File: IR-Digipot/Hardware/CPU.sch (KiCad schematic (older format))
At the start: 14 parts, among them J1 Conn_1x06_Generic, J2 Conn_1x03_Generic, U1 PIC18F2550T-I/SO, U2 TCM809, U3 TSOP754, X1 20 MHz

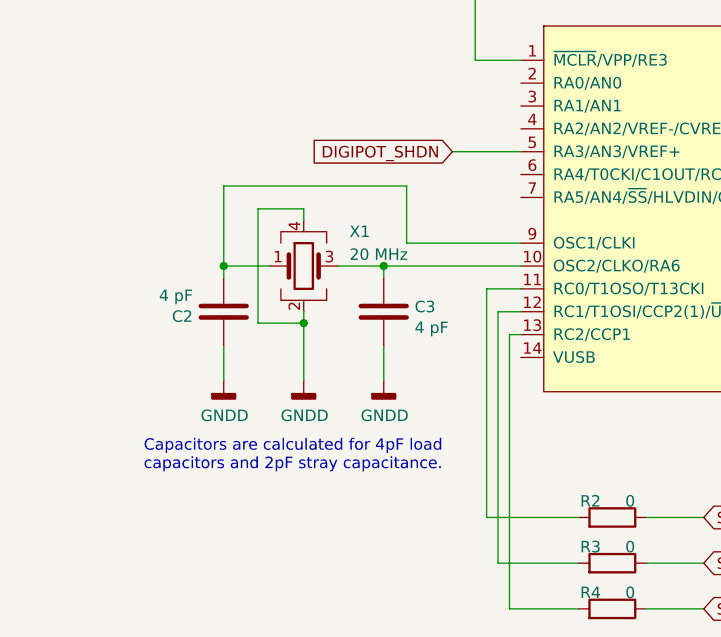
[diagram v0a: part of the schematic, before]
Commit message: Wire high-side switch FET for +5VA
The PIC port should be able to draw enough current to
properly control the switch.
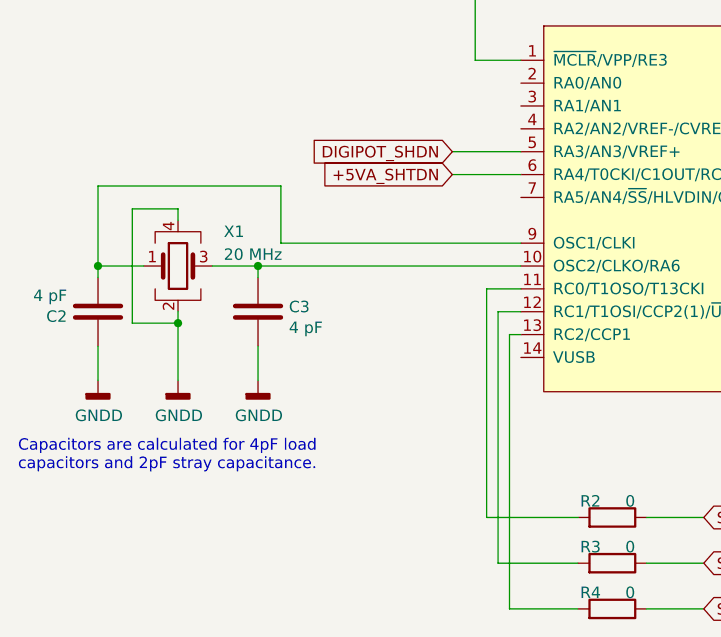
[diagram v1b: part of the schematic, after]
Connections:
- net +5VA_SHTDN: now reaches U1.6 (RA4/T0CKI/C1OUT/RCV)
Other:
- moved on the sheet: C2, C3, X1
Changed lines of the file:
@@
 L Library:Crystal_GND24 X1
 U 1 1 5FE286DC
-P 2300 3600
-F 0 "X1" H 2500 3750 50  0000 L CNN
-F 1 "20 MHz" H 2500 3650 50  0000 L CNN
-F 2 "Librray:Crystal_SMD_4Pin_3.2x2.5mm" H 2700 3600 50  0001 C CNN
-F 3 "${KIPRJMOD}/../../Datasheet/ABM10W SERIES IoT OPTIMIZED LOW PROFILE QUARTZ CRYSTAL.pdf" H 2700 3600 50  0001 C CNN
-F 4 "CRYSTAL 20.0000MHZ 4PF SMD" H 2300 3600 50  0001 C CNN "Description"
-F 5 "Abracon LLC" H 2300 3600 50  0001 C CNN "Manufacturer"
-F 6 "ABM8W-20.0000MHZ-4-K1Z-T3" H 2300 3600 50  0001 C CNN "Manufacturer Part Number"
-F 7 "535-14037-1-ND" H 2300 3600 50  0001 C CNN "Digi-Key Part Number"
-	1    2300 3600
-	1    0    0    -1
-$EndComp
-Wire Wire Line
-	3250 3500 2750 3500
-Wire Wire Line
-	2750 3500 2750 3250
+P 1750 3600
+F 0 "X1" H 1950 3750 50  0000 L CNN
+F 1 "20 MHz" H 1950 3650 50  0000 L CNN
+F 2 "Librray:Crystal_SMD_4Pin_3.2x2.5mm" H 2150 3600 50  0001 C CNN
+F 3 "${KIPRJMOD}/../../Datasheet/ABM10W SERIES IoT OPTIMIZED LOW PROFILE QUARTZ CRYSTAL.pdf" H 2150 3600 50  0001 C CNN
+F 4 "CRYSTAL 20.0000MHZ 4PF SMD" H 1750 3600 50  0001 C CNN "Description"
+F 5 "Abracon LLC" H 1750 3600 50  0001 C CNN "Manufacturer"
+F 6 "ABM8W-20.0000MHZ-4-K1Z-T3" H 1750 3600 50  0001 C CNN "Manufacturer Part Number"
+F 7 "535-14037-1-ND" H 1750 3600 50  0001 C CNN "Digi-Key Part Number"
+	1    1750 3600
+	1    0    0    -1
+$EndComp
+Wire Wire Line
+	2200 3500 2200 3250
 $Comp
 L Library:C C3
 U 1 1 5FE2C5B6
-P 2650 3800
-F 0 "C3" V 2671 3665 50  0000 R CNN
-F 1 "4 pF" V 2580 3665 50  0000 R CNN
-F 2 "Librray:C_0402_1005Metric" H 2500 4000 50  0001 C CNN
-F 3 "" H 2500 4000 50  0001 C CNN
-F 4 "CAP CER 4PF 50V C0G/NP0 0402" V 2650 3800 50  0001 C CNN "Description"
-F 5 "KEMET" V 2650 3800 50  0001 C CNN "Manufacturer"
-F 6 "CBR04C409B5GAC" V 2650 3800 50  0001 C CNN "Manufacturer Part Number"
-F 7 "399-13246-1-ND" V 2650 3800 50  0001 C CNN "Digi-Key Part Number"
-	1    2650 3800
+P 2100 3800
+F 0 "C3" V 2121 3665 50  0000 R CNN
+F 1 "4 pF" V 2030 3665 50  0000 R CNN
+F 2 "Librray:C_0402_1005Metric" H 1950 4000 50  0001 C CNN
+F 3 "" H 1950 4000 50  0001 C CNN
+F 4 "CAP CER 4PF 50V C0G/NP0 0402" V 2100 3800 50  0001 C CNN "Description"
+F 5 "KEMET" V 2100 3800 50  0001 C CNN "Manufacturer"
+F 6 "CBR04C409B5GAC" V 2100 3800 50  0001 C CNN "Manufacturer Part Number"
+F 7 "399-13246-1-ND" V 2100 3800 50  0001 C CNN "Digi-Key Part Number"
+	1    2100 3800
 	0    -1   -1   0
 $EndComp
@@
 L power:GNDD #PWR05
 U 1 1 5FE2F103
-P 2650 4100
-F 0 "#PWR05" H 2650 3850 50  0001 C CNN
-F 1 "GNDD" H 2654 3945 50  0000 C CNN
-F 2 "" H 2650 4100 50  0001 C CNN
-F 3 "" H 2650 4100 50  0001 C CNN
-	1    2650 4100
+P 2100 4100
+F 0 "#PWR05" H 2100 3850 50  0001 C CNN
+F 1 "GNDD" H 2104 3945 50  0000 C CNN
+F 2 "" H 2100 4100 50  0001 C CNN
+F 3 "" H 2100 4100 50  0001 C CNN
+	1    2100 4100
 	1    0    0    -1
 $EndComp
@@
 L power:GNDD #PWR03
 U 1 1 5FE2F5E3
-P 1950 4100
-F 0 "#PWR03" H 1950 3850 50  0001 C CNN
-F 1 "GNDD" H 1954 3945 50  0000 C CNN
-F 2 "" H 1950 4100 50  0001 C CNN
-F 3 "" H 1950 4100 50  0001 C CNN
-	1    1950 4100
+P 1400 4100
+F 0 "#PWR03" H 1400 3850 50  0001 C CNN
+F 1 "GNDD" H 1404 3945 50  0000 C CNN
+F 2 "" H 1400 4100 50  0001 C CNN
+F 3 "" H 1400 4100 50  0001 C CNN
+	1    1400 4100
 	1    0    0    -1
 $EndComp
@@
 L power:GNDD #PWR04
 U 1 1 5FE2FF95
-P 2300 4100
-F 0 "#PWR04" H 2300 3850 50  0001 C CNN
-F 1 "GNDD" H 2304 3945 50  0000 C CNN
-F 2 "" H 2300 4100 50  0001 C CNN
-F 3 "" H 2300 4100 50  0001 C CNN
-	1    2300 4100
-	1    0    0    -1
-$EndComp
-Wire Wire Line
-	2450 3600 2650 3600
-Wire Wire Line
-	2300 3800 2300 3850
-Wire Wire Line
-	2100 3350 2100 3850
-Wire Wire Line
-	2100 3850 2300 3850
-Wire Wire Line
-	2100 3350 2300 3350
-Connection ~ 2300 3850
-Wire Wire Line
-	2300 3850 2300 4100
-Wire Wire Line
-	1950 3600 1950 3650
-Wire Wire Line
-	1950 3600 2150 3600
-Wire Wire Line
-	1950 3600 1950 3250
-Wire Wire Line
-	1950 3250 2750 3250
-Connection ~ 1950 3600
-Wire Wire Line
-	2650 3650 2650 3600
-Connection ~ 2650 3600
-Wire Wire Line
-	2650 3600 3250 3600
-Wire Wire Line
-	2300 3350 2300 3400
-Text Notes 1600 4500 0    50   ~ 0
+P 1750 4100
+F 0 "#PWR04" H 1750 3850 50  0001 C CNN
+F 1 "GNDD" H 1754 3945 50  0000 C CNN
+F 2 "" H 1750 4100 50  0001 C CNN
+F 3 "" H 1750 4100 50  0001 C CNN
+	1    1750 4100
+	1    0    0    -1
+$EndComp
+Wire Wire Line
+	1900 3600 2100 3600
+Wire Wire Line
+	1750 3800 1750 3850
+Wire Wire Line
+	1550 3350 1550 3850
+Wire Wire Line
+	1550 3850 1750 3850
+Wire Wire Line
+	1550 3350 1750 3350
+Connection ~ 1750 3850
+Wire Wire Line
+	1750 3850 1750 4100
+Wire Wire Line
+	1400 3600 1400 3650
+Wire Wire Line
+	1400 3600 1600 3600
+Wire Wire Line
+	1400 3600 1400 3250
+Wire Wire Line
+	1400 3250 2200 3250
+Connection ~ 1400 3600
+Wire Wire Line
+	2100 3650 2100 3600
+Connection ~ 2100 3600
+Wire Wire Line
+	1750 3350 1750 3400
+Text Notes 1050 4500 0    50   ~ 0
 Capacitors are calculated for 4pF load\ncapacitors and 2pF stray capacitance.
 $Comp
@@
 L Library:C C2
 U 1 1 5FE2B3B5
-P 1950 3800
-F 0 "C2" V 1971 3665 50  0000 R CNN
-F 1 "4 pF" V 1880 3665 50  0000 R CNN
-F 2 "Librray:C_0402_1005Metric" H 1800 4000 50  0001 C CNN
-F 3 "" H 1800 4000 50  0001 C CNN
-F 4 "CAP CER 4PF 50V C0G/NP0 0402" V 1950 3800 50  0001 C CNN "Description"
-F 5 "KEMET" V 1950 3800 50  0001 C CNN "Manufacturer"
-F 6 "CBR04C409B5GAC" V 1950 3800 50  0001 C CNN "Manufacturer Part Number"
-F 7 "399-13246-1-ND" V 1950 3800 50  0001 C CNN "Digi-Key Part Number"
-	1    1950 3800
+P 1400 3800
+F 0 "C2" V 1421 3665 50  0000 R CNN
+F 1 "4 pF" V 1330 3665 50  0000 R CNN
+F 2 "Librray:C_0402_1005Metric" H 1250 4000 50  0001 C CNN
+F 3 "" H 1250 4000 50  0001 C CNN
+F 4 "CAP CER 4PF 50V C0G/NP0 0402" V 1400 3800 50  0001 C CNN "Description"
+F 5 "KEMET" V 1400 3800 50  0001 C CNN "Manufacturer"
+F 6 "CBR04C409B5GAC" V 1400 3800 50  0001 C CNN "Manufacturer Part Number"
+F 7 "399-13246-1-ND" V 1400 3800 50  0001 C CNN "Digi-Key Part Number"
+	1    1400 3800
 	0    1    1    0
 $EndComp
 Wire Wire Line
-	2650 3950 2650 4100
-Wire Wire Line
-	1950 3950 1950 4100
+	2100 3950 2100 4100
+Wire Wire Line
+	1400 3950 1400 4100
 Wire Wire Line
 	7500 5100 7500 5150
@@
 Wire Wire Line
 	3100 4700 3500 4700
+Wire Wire Line
+	2200 3500 3250 3500
+Wire Wire Line
+	2100 3600 3250 3600
+Text GLabel 2950 3200 0    50   Input ~ 0
++5VA_SHTDN
+Wire Wire Line
+	2950 3200 3250 3200
 $EndSCHEMATC

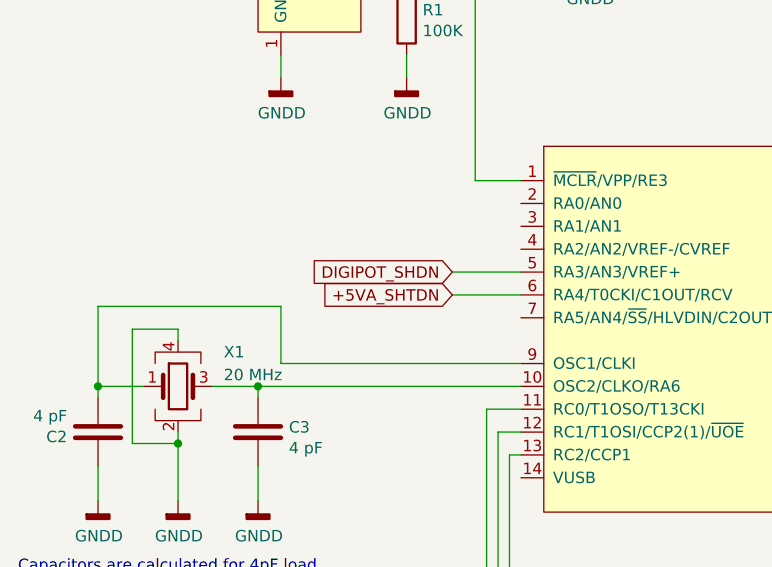
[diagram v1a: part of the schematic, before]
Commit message: Continue routing digipot receiver
Minor touches to the USB-C PD tracks, routed signal paths of
audio circuits.

Added missing reset circuits for the digipot.
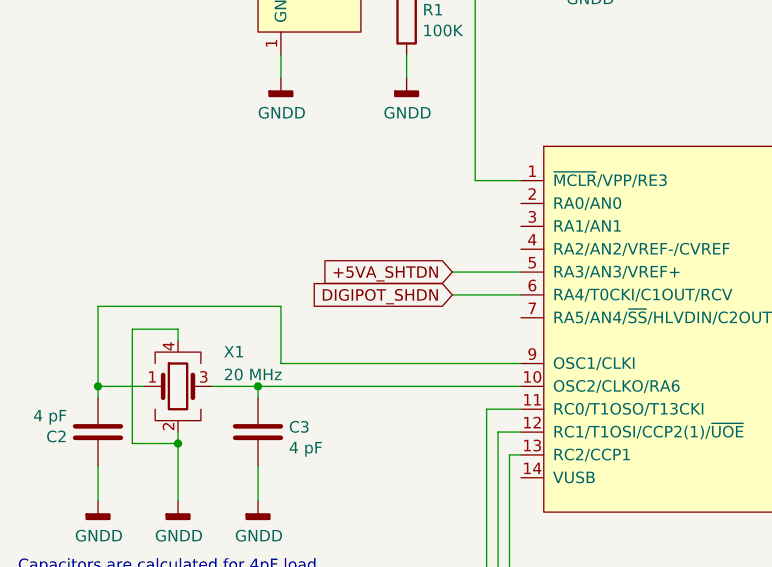
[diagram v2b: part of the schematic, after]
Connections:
- net +5VA_SHTDN: now also U1.5 (RA3/AN3/VREF+); no longer U1.6 (RA4/T0CKI/C1OUT/RCV)
- net DIGIPOT_SHDN: now also U1.6 (RA4/T0CKI/C1OUT/RCV); no longer U1.5 (RA3/AN3/VREF+)
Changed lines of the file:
@@
 	6050 2800 6800 2800
-$Comp
-L Library:Conn_1x03_Generic J2
-U 1 1 5FE58490
-P 6950 3600
-F 0 "J2" H 7078 3451 50  0000 L CNN
-F 1 "Conn_1x03_Generic" H 7078 3360 50  0000 L CNN
-F 2 "Librray:Conn_1x03_D0.65mm_Pitch2.54mm_staggered" H 6950 3600 50  0001 C CNN
-F 3 "" H 6950 3600 50  0001 C CNN
-	1    6950 3600
-	1    0    0    -1
-$EndComp
-Wire Wire Line
-	6050 3700 6800 3700
-Wire Wire Line
-	6050 3800 6800 3800
-$Comp
-L power:GNDD #PWR06
-U 1 1 5FE5ACFD
-P 6750 4000
-F 0 "#PWR06" H 6750 3750 50  0001 C CNN
-F 1 "GNDD" H 6754 3845 50  0000 C CNN
-F 2 "" H 6750 4000 50  0001 C CNN
-F 3 "" H 6750 4000 50  0001 C CNN
-	1    6750 4000
-	1    0    0    -1
-$EndComp
-Wire Wire Line
-	6750 4000 6750 3900
-Wire Wire Line
-	6750 3900 6800 3900
-Text Notes 6900 3600 0    50   ~ 0
-UART
 $Comp
 L Library:TSOP754 U3
@@
 Text GLabel 4050 5100 2    50   Input ~ 0
 SPI_MOSI
-Text GLabel 2950 3100 0    50   Input ~ 0
-DIGIPOT_SHDN
 Wire Wire Line
 	2950 3100 3250 3100
@@
 	2100 3600 3250 3600
 Text GLabel 2950 3200 0    50   Input ~ 0
+DIGIPOT_SHDN
+Text Notes 6900 3600 0    50   ~ 0
+UART
+Wire Wire Line
+	6750 3900 6800 3900
+Wire Wire Line
+	6750 4000 6750 3900
+$Comp
+L power:GNDD #PWR06
+U 1 1 5FE5ACFD
+P 6750 4000
+F 0 "#PWR06" H 6750 3750 50  0001 C CNN
+F 1 "GNDD" H 6754 3845 50  0000 C CNN
+F 2 "" H 6750 4000 50  0001 C CNN
+F 3 "" H 6750 4000 50  0001 C CNN
+	1    6750 4000
+	1    0    0    -1
+$EndComp
+Wire Wire Line
+	6050 3800 6800 3800
+Wire Wire Line
+	6050 3700 6800 3700
+$Comp
+L Library:Conn_1x03_Generic J2
+U 1 1 5FE58490
+P 6950 3600
+F 0 "J2" H 7078 3451 50  0000 L CNN
+F 1 "Conn_1x03_Generic" H 7078 3360 50  0000 L CNN
+F 2 "Librray:Conn_1x03_D0.65mm_Pitch2.54mm_staggered" H 6950 3600 50  0001 C CNN
+F 3 "" H 6950 3600 50  0001 C CNN
+	1    6950 3600
+	1    0    0    -1
+$EndComp
+Text GLabel 2950 3100 0    50   Input ~ 0
 +5VA_SHTDN
 Wire Wire Line
